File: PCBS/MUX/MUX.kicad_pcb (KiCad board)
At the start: 2 copper layers, 30 x 15 mm, 17 parts, among them J1 Conn_01x01_Socket, J2 Conn_01x01_Socket, J3 Conn_01x03_Socket, J6 Conn_01x01_Socket, U1 SN74LVC2G157DCTR

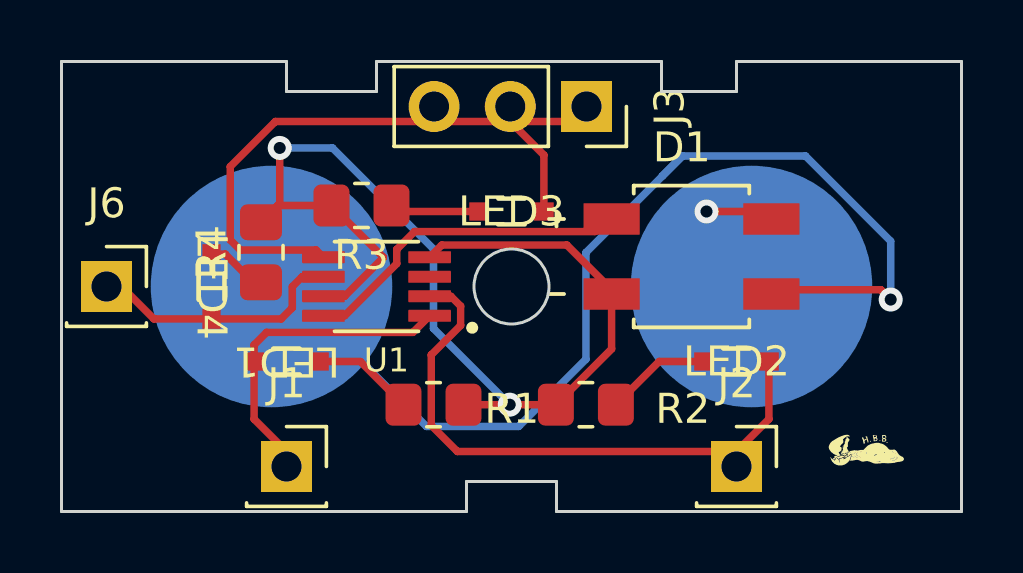
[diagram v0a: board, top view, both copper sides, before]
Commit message: Rev1 board/mux/switches/output
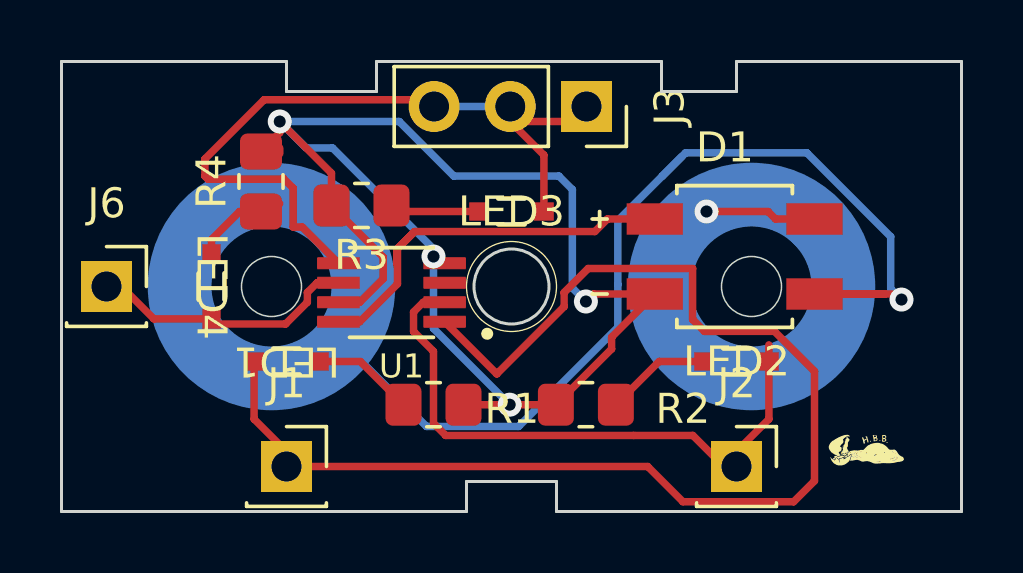
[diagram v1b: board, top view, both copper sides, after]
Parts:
- added G***: LOGO, DigitalLogicFootprints:HBBLogo, B.Cu at (165.1, 93.5)
- moved R4 2.36 mm to (146.7, 84.0)
- moved D1 1.44 mm to (162.4, 86.5)
- moved U1 0.54 mm to (151.0, 87.7)
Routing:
- net Net-(J1-Pin_1): track 10.3 -> 42.7 mm
- net GND: track 37.6 -> 48.7 mm, vias 2 -> 4
- net Net-(J5-PWR): track 5.12 -> 9.24 mm
- net VCC: track 11.3 -> 14.0 mm
- net Net-(J3-Pin_1): track 21.7 -> 24.1 mm
- net Net-(LED4-Pad1): track 2.04 -> 4.20 mm
- net Net-(J4-PWR): track 36.1 -> 36.6 mm
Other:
- board text added: "Jonathan Hess (jetsama.com)"
- board text added: "Mux PCB Rev 1"
